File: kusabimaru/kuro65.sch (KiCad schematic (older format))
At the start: 23 parts, among them IC1 ATMEGA32U4, J1 ISP, J2 USB4085-GF-A, SW1 SW_RESET, Y1 16MHz

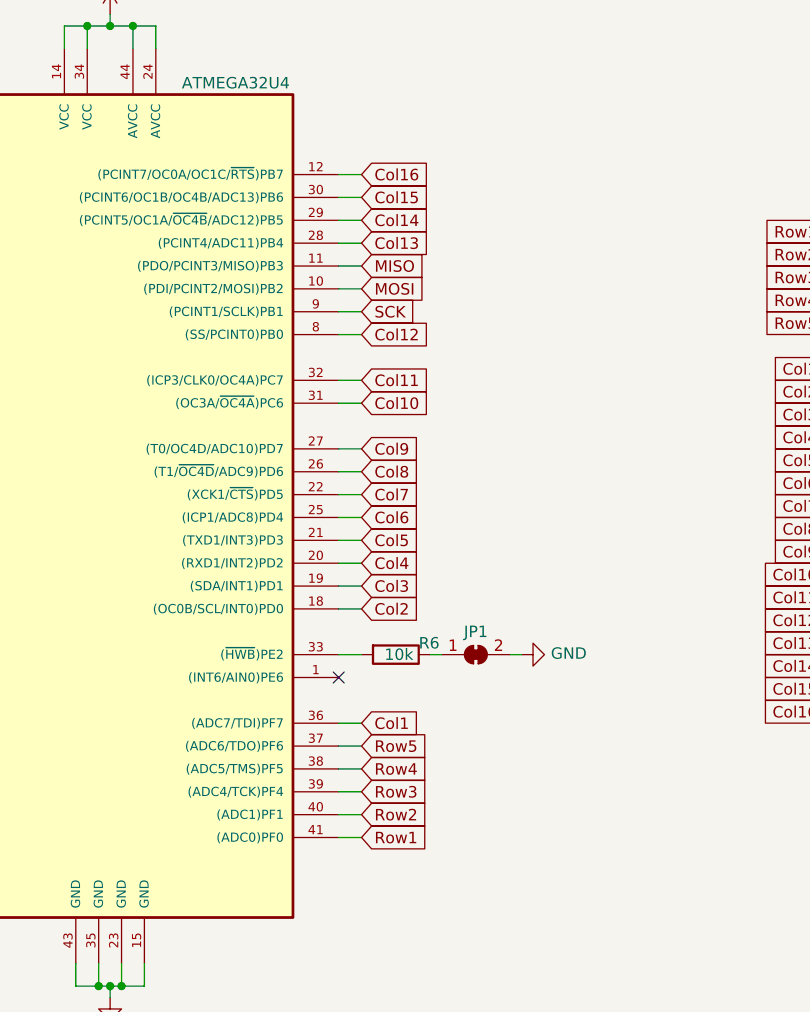
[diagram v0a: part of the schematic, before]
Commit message: Routing completed. Some modifications still needed.
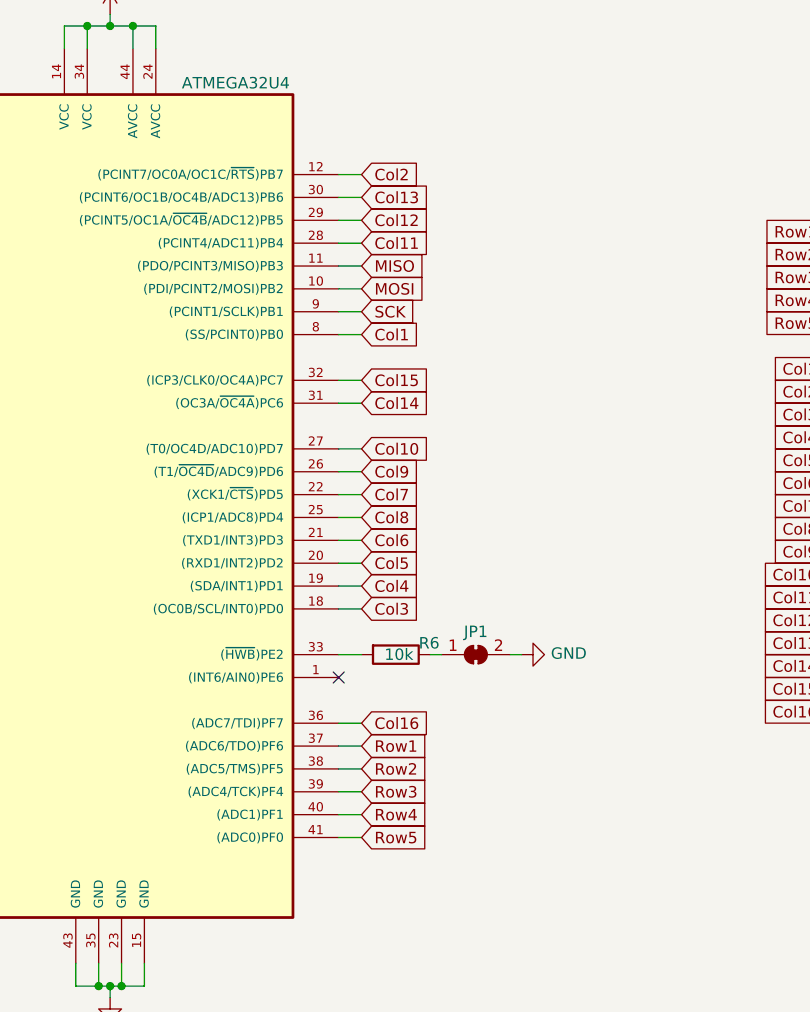
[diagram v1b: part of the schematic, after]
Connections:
- net Col1: now also IC1.8 ((SS/PCINT0)PB0); no longer IC1.36 ((ADC7/TDI)PF7)
- net Col10: now also IC1.27 ((T0/OC4D/ADC10)PD7); no longer IC1.31 ((OC3A/~OC4A~)PC6)
- net Col11: now also IC1.28 ((PCINT4/ADC11)PB4); no longer IC1.32 ((ICP3/CLK0/OC4A)PC7)
- net Col12: now also IC1.29 ((PCINT5/OC1A/~OC4B~/ADC12)PB5); no longer IC1.8 ((SS/PCINT0)PB0)
- net Col13: now also IC1.30 ((PCINT6/OC1B/OC4B/ADC13)PB6); no longer IC1.28 ((PCINT4/ADC11)PB4)
- net Col14: now also IC1.31 ((OC3A/~OC4A~)PC6); no longer IC1.29 ((PCINT5/OC1A/~OC4B~/ADC12)PB5)
- net Col15: now also IC1.32 ((ICP3/CLK0/OC4A)PC7); no longer IC1.30 ((PCINT6/OC1B/OC4B/ADC13)PB6)
- net Col16: now also IC1.36 ((ADC7/TDI)PF7); no longer IC1.12 ((PCINT7/OC0A/OC1C/~RTS~)PB7)
- net Col2: now also IC1.12 ((PCINT7/OC0A/OC1C/~RTS~)PB7); no longer IC1.18 ((OC0B/SCL/INT0)PD0)
- net Col3: now also IC1.18 ((OC0B/SCL/INT0)PD0); no longer IC1.19 ((SDA/INT1)PD1)
- net Col4: now also IC1.19 ((SDA/INT1)PD1); no longer IC1.20 ((RXD1/INT2)PD2)
- net Col5: now also IC1.20 ((RXD1/INT2)PD2); no longer IC1.21 ((TXD1/INT3)PD3)
- net Col6: now also IC1.21 ((TXD1/INT3)PD3); no longer IC1.25 ((ICP1/ADC8)PD4)
- net Col8: now also IC1.25 ((ICP1/ADC8)PD4); no longer IC1.26 ((T1/~OC4D~/ADC9)PD6)
- net Col9: now also IC1.26 ((T1/~OC4D~/ADC9)PD6); no longer IC1.27 ((T0/OC4D/ADC10)PD7)
- net Row1: now also IC1.37 ((ADC6/TDO)PF6); no longer IC1.41 ((ADC0)PF0)
- net Row2: now also IC1.38 ((ADC5/TMS)PF5); no longer IC1.40 ((ADC1)PF1)
- net Row4: now also IC1.40 ((ADC1)PF1); no longer IC1.38 ((ADC5/TMS)PF5)
- net Row5: now also IC1.41 ((ADC0)PF0); no longer IC1.37 ((ADC6/TDO)PF6)
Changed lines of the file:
@@
 F22 "Col16" I L 7850 4100 50
 $EndSheet
-Text GLabel 5700 4650 2    50   Input ~ 0
+Text GLabel 5700 4250 2    50   Input ~ 0
 Row1
-Text GLabel 5700 4550 2    50   Input ~ 0
+Text GLabel 5700 4350 2    50   Input ~ 0
 Row2
 Text GLabel 5700 4450 2    50   Input ~ 0
 Row3
-Text GLabel 5700 4350 2    50   Input ~ 0
+Text GLabel 5700 4550 2    50   Input ~ 0
 Row4
-Text GLabel 5700 4250 2    50   Input ~ 0
+Text GLabel 5700 4650 2    50   Input ~ 0
 Row5
 Wire Wire Line
@@
 Wire Wire Line
 	7850 2000 7750 2000
-Text GLabel 5700 4150 2    50   Input ~ 0
+Text GLabel 5700 2450 2    50   Input ~ 0
 Col1
+Text GLabel 5700 1750 2    50   Input ~ 0
+Col2
 Text GLabel 5700 3650 2    50   Input ~ 0
-Col2
+Col3
 Text GLabel 5700 3550 2    50   Input ~ 0
-Col3
+Col4
 Text GLabel 5700 3450 2    50   Input ~ 0
-Col4
+Col5
 Text GLabel 5700 3350 2    50   Input ~ 0
-Col5
-Text GLabel 5700 3250 2    50   Input ~ 0
 Col6
 Text GLabel 5700 3150 2    50   Input ~ 0
 Col7
+Text GLabel 5700 3250 2    50   Input ~ 0
+Col8
 Text GLabel 5700 3050 2    50   Input ~ 0
-Col8
+Col9
 Text GLabel 5700 2950 2    50   Input ~ 0
-Col9
+Col10
+Text GLabel 5700 2050 2    50   Input ~ 0
+Col11
+Text GLabel 5700 1950 2    50   Input ~ 0
+Col12
+Text GLabel 5700 1850 2    50   Input ~ 0
+Col13
 Text GLabel 5700 2750 2    50   Input ~ 0
-Col10
+Col14
 Text GLabel 5700 2650 2    50   Input ~ 0
-Col11
-Text GLabel 5700 2450 2    50   Input ~ 0
-Col12
-Text GLabel 5700 2050 2    50   Input ~ 0
-Col13
-Text GLabel 5700 1950 2    50   Input ~ 0
-Col14
-Text GLabel 5700 1850 2    50   Input ~ 0
 Col15
-Text GLabel 5700 1750 2    50   Input ~ 0
+Text GLabel 5700 4150 2    50   Input ~ 0
 Col16
 Wire Wire Line
